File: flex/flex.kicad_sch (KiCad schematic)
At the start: 28 parts, among them J1 Conn_01x06_Female, J2 Conn_01x03_Female, J3 Conn_01x01_Female, SW1 SW_Push, SW14 SW_Push, SW19 SW_Push, SW5 SW_Push, SW9 SW_Push

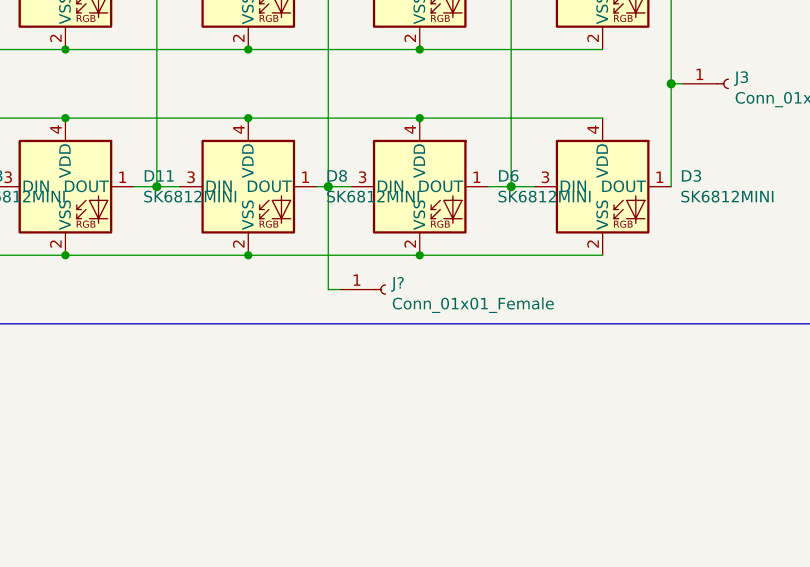
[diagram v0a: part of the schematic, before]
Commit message: drc
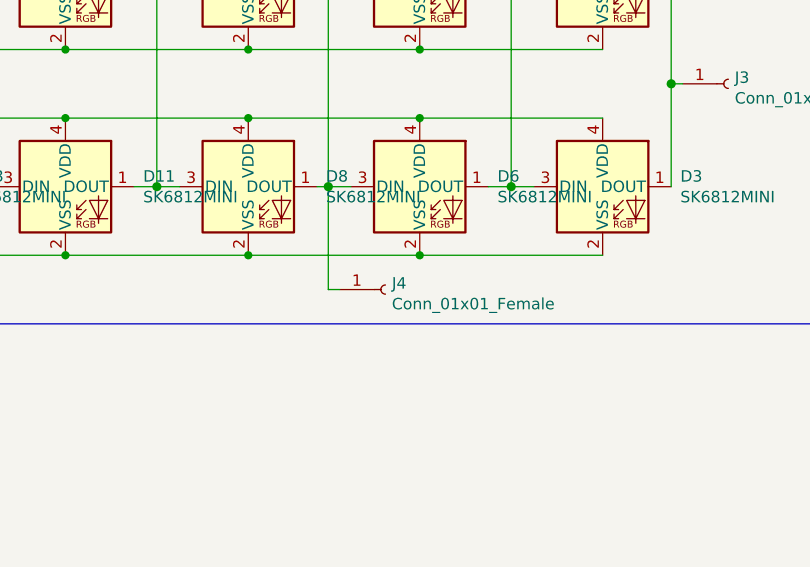
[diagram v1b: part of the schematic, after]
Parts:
- J3: footprint Connector_PinHeader_2.54mm:PinHeader_1x01_P2.54mm_Vertical -> custom:PinHeader_1x01_P2.54mm_Vertical
- J4: renamed from J?; footprint Connector_PinHeader_2.54mm:PinHeader_1x01_P2.54mm_Vertical -> custom:PinHeader_1x01_P2.54mm_Vertical
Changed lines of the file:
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@@
   (symbol (lib_id "Connector:Conn_01x01_Female") (at 151.13 114.3 0) (unit 1)
     (in_bom yes) (on_board yes)
-    (property "Reference" "J?" (id 0) (at 151.8413 113.6078 0)
+    (property "Reference" "J4" (id 0) (at 151.8413 113.6078 0)
       (effects (font (size 1.27 1.27)) (justify left))
     )
@@
       (effects (font (size 1.27 1.27)) (justify left))
     )
-    (property "Footprint" "Connector_PinHeader_2.54mm:PinHeader_1x01_P2.54mm_Vertical" (id 2) (at 151.13 114.3 0)
+    (property "Footprint" "custom:PinHeader_1x01_P2.54mm_Vertical" (id 2) (at 151.13 114.3 0)
       (effects (font (size 1.27 1.27)) hide)
     )
@@
       (effects (font (size 1.27 1.27)) (justify left))
     )
-    (property "Footprint" "Connector_PinHeader_2.54mm:PinHeader_1x01_P2.54mm_Vertical" (id 2) (at 189.23 91.44 0)
+    (property "Footprint" "custom:PinHeader_1x01_P2.54mm_Vertical" (id 2) (at 189.23 91.44 0)
       (effects (font (size 1.27 1.27)) hide)
     )
@@
     )
     (path "/d7dd6422-5a2c-4c20-8c63-6ad26180679c"
-      (reference "J3") (unit 1) (value "Conn_01x01_Female") (footprint "Connector_PinHeader_2.54mm:PinHeader_1x01_P2.54mm_Vertical")
+      (reference "J3") (unit 1) (value "Conn_01x01_Female") (footprint "custom:PinHeader_1x01_P2.54mm_Vertical")
     )
     (path "/53891b88-f1a1-4c61-b083-3fcaa127f940"
-      (reference "J?") (unit 1) (value "Conn_01x01_Female") (footprint "Connector_PinHeader_2.54mm:PinHeader_1x01_P2.54mm_Vertical")
+      (reference "J4") (unit 1) (value "Conn_01x01_Female") (footprint "custom:PinHeader_1x01_P2.54mm_Vertical")
     )
     (path "/6254aa13-411d-4aa6-a1ef-3424dce5a979"
